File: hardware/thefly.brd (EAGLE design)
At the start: 54 x 54 mm, 31 parts, among them IC1 AP7313-1.8, J1 54-00298, U1 SGTL5000XNLA3, U2 MAX4466EXK

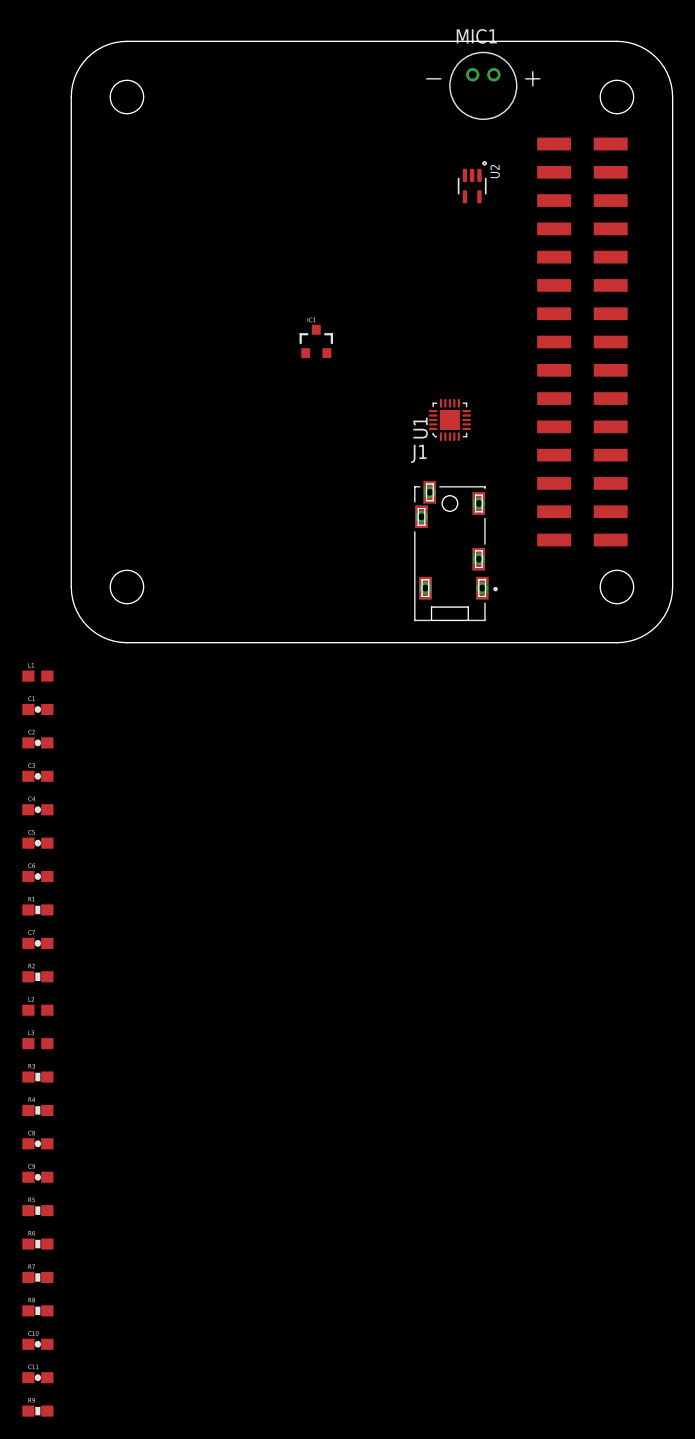
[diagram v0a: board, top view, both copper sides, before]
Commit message: elec layout progress
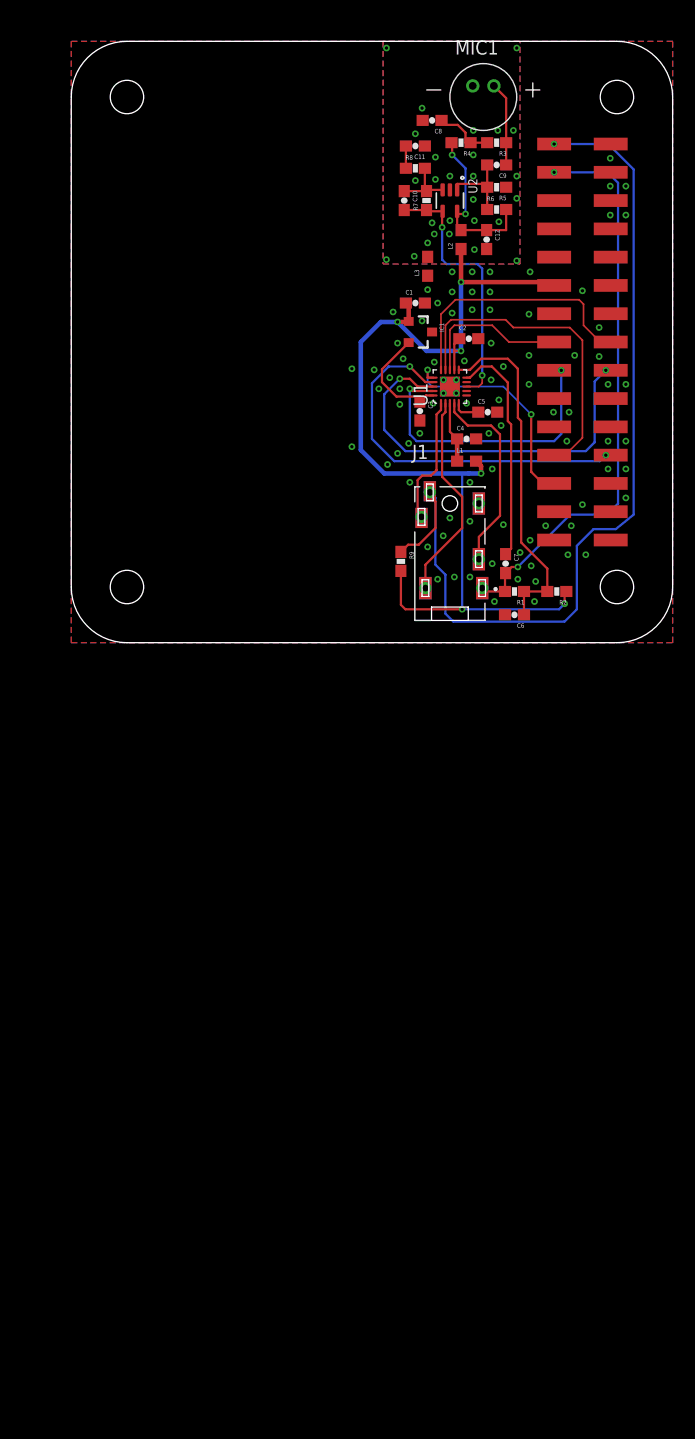
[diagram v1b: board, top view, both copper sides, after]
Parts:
- added C12: 100n, thefly:0603-CAP
- moved C11 115.7 mm to (30.9, 44.6), turned to 180 degrees
- moved R8 108.1 mm to (30.9, 42.6)
- moved C10 107.8 mm to (29.9, 39.7), turned to 270 degrees
- moved R7 102.8 mm to (31.9, 39.7), turned to 90 degrees
- moved R6 101.6 mm to (38.2, 38.9)
- moved R5 100.7 mm to (38.2, 40.9), turned to 180 degrees
- moved C9 99.8 mm to (38.2, 42.9), turned to 180 degrees
- moved C8 98.5 mm to (32.4, 46.9), turned to 180 degrees
- moved R4 94.8 mm to (35.0, 44.9), turned to 180 degrees
- moved R3 93.5 mm to (38.2, 44.9), turned to 180 degrees
- moved R9 83.0 mm to (29.6, 7.30), turned to 270 degrees
- moved L2 78.9 mm to (35.0, 36.2), turned to 90 degrees
- moved L3 78.1 mm to (32.0, 33.8), turned to 90 degrees
- moved R2 58.0 mm to (43.6, 4.60), turned to 180 degrees
- moved C5 55.9 mm to (37.4, 20.7)
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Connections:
- net AGND: now also C12.2
- net BCLK: now also JP1.15; no longer JP1.21
- net HP-L: now also U1.1; no longer U1.4
- net HP-R: now also U1.4; no longer U1.1
- net MCLK: now also JP1.16; no longer JP1.19
- net N$2: now also C12.1
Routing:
- net 3.3V: track 0.00 -> 90.0 mm, vias 0 -> 6
- net HP-SENSE-L: track 0.00 -> 82.4 mm, vias 0 -> 1
- net HP-MIC: track 0.00 -> 51.7 mm, vias 0 -> 2
- net SDA: track 0.00 -> 35.8 mm, vias 0 -> 2
- net I2S_DIN: track 0.00 -> 34.2 mm, vias 0 -> 2
- net N$4: track 0.00 -> 31.4 mm
- net LRCLK: track 0.00 -> 29.2 mm
- net SCL: track 0.00 -> 26.8 mm, vias 0 -> 2
- net MIC2: track 0.00 -> 23.6 mm, vias 0 -> 2
- net BCLK: track 0.00 -> 23.5 mm
- net N$5: track 0.00 -> 20.5 mm
- net I2S_DOUT: track 0.00 -> 20.4 mm, vias 0 -> 2
- net HP-GND: track 0.00 -> 18.8 mm
- net HP-R: track 0.00 -> 17.7 mm
- net N$2: track 0.00 -> 15.7 mm, vias 0 -> 2
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- added copper zone on layer 1, net AGND
- added copper zone on layer 16, net AGND
- added copper zone on layer 1, net GND
- added copper zone on layer 16, net GND
